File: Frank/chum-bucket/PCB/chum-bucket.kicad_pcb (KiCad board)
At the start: 4 copper layers, 130.7 x 220 mm, 300 parts, among them J1 Conn_01x02, J2 Conn_01x02, J205 CAN_CONN, J206 SWD_DIAGS, J3 Conn_01x02, J7 ESC_PWR, J8 ESC_GND, Q101 2N7002K, Q102 BSS84, Q301 AON2406, Q302 AON2406, Q303 AON2406, Q401 BSS84, Q402 2N7002K, Q403 Q_NMOS_DGS, SW201 B3U-1000P, SW202 LV_EN, SW203 B3U-1000P, U1 INA194, U100 BTS6142DAUMA1, U101 BQ2461x, U102 INA196, U103 CSD87331, U2 SN65HVD232, U215 STM32F042K6Tx, U216 TPS70933DRVT, U301 BQ79606, U401 SN74LVC1G08DRYR, U402 MCP6241-E, U403 NCP81080, U404 MP5000ADQ, Y201 XTAL

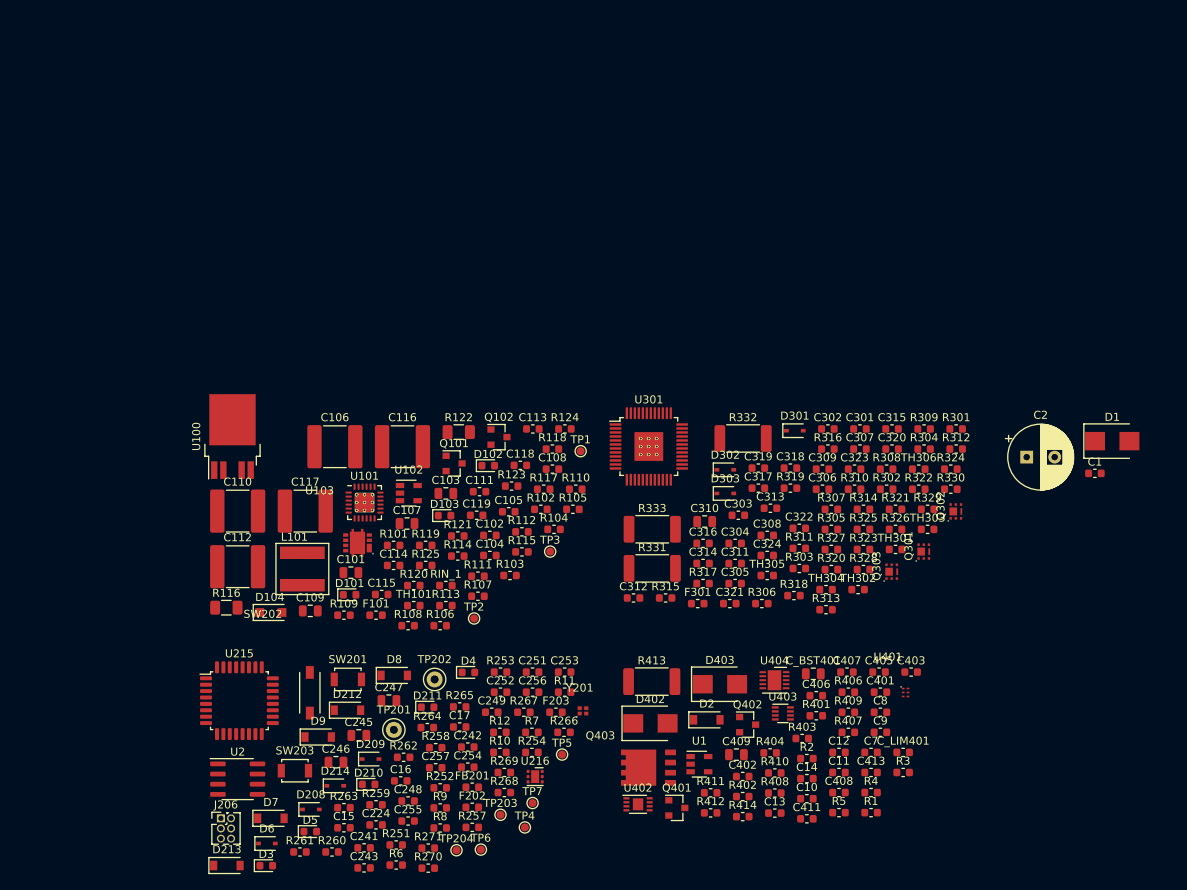
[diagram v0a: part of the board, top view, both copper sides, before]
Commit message: First Official Schematic Release
yeet
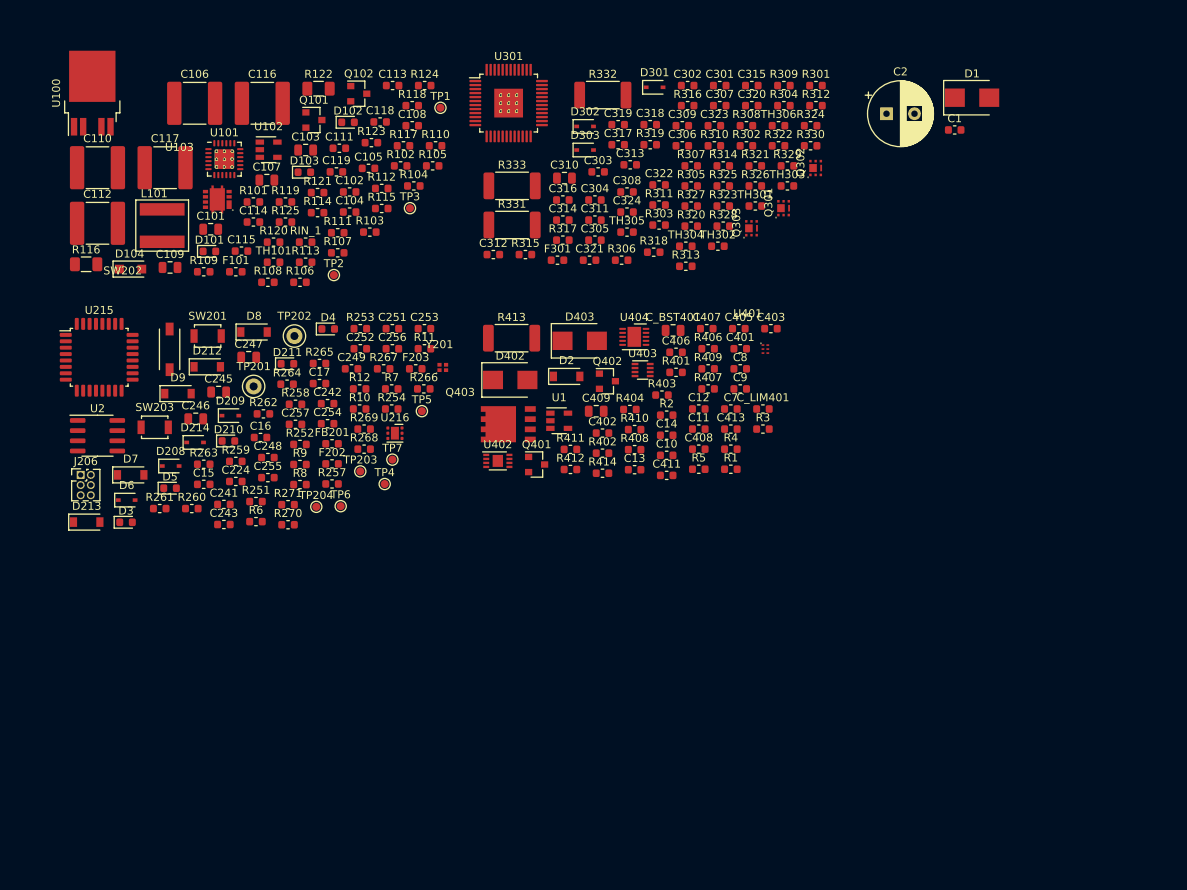
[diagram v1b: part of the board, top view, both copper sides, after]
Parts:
- moved C103 46.4 mm to (133.1, 273.7)
- moved C104 46.4 mm to (138.6, 281.4)
- moved C107 46.4 mm to (128.2, 277.4)
- moved C113 46.4 mm to (144.0, 265.6)
- moved C114 46.4 mm to (126.6, 282.7)
- moved C115 46.4 mm to (125.1, 286.3)
- moved C17 46.4 mm to (134.8, 302.9)
- moved C245 46.4 mm to (122.2, 303.9)
- moved C248 46.4 mm to (128.4, 312.1)
- moved C301 46.4 mm to (184.9, 265.6)
- moved C302 46.4 mm to (180.8, 265.6)
- moved C305 46.4 mm to (169.3, 284.9)
- moved C310 46.4 mm to (165.4, 277.2)
- moved C311 46.4 mm to (169.3, 282.4)
- moved C314 46.4 mm to (165.2, 282.4)
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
